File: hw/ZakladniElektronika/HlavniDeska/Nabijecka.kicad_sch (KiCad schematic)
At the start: 1 part

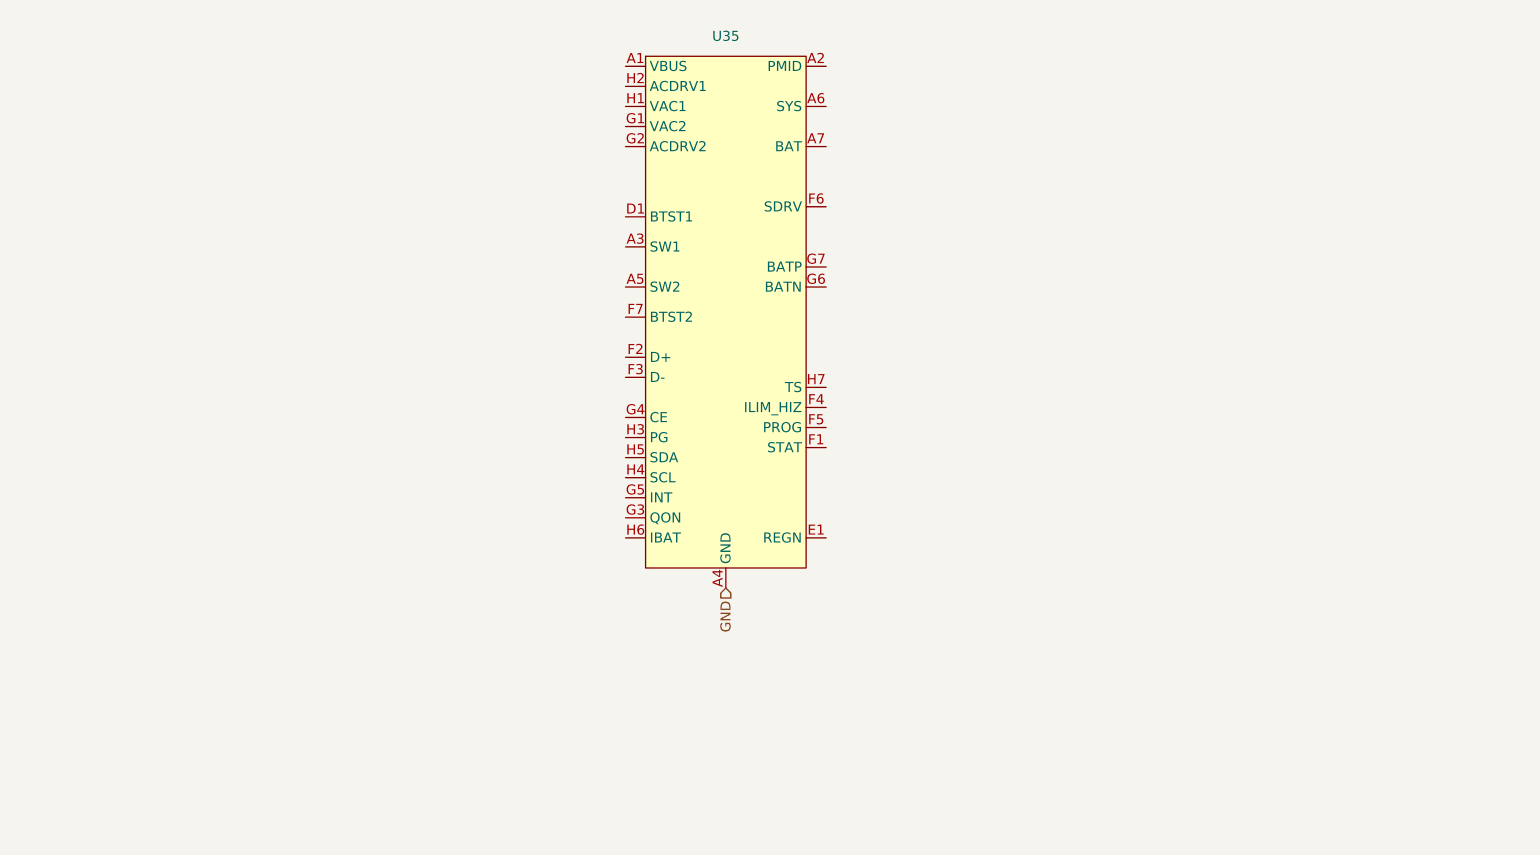
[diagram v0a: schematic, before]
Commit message: WIP
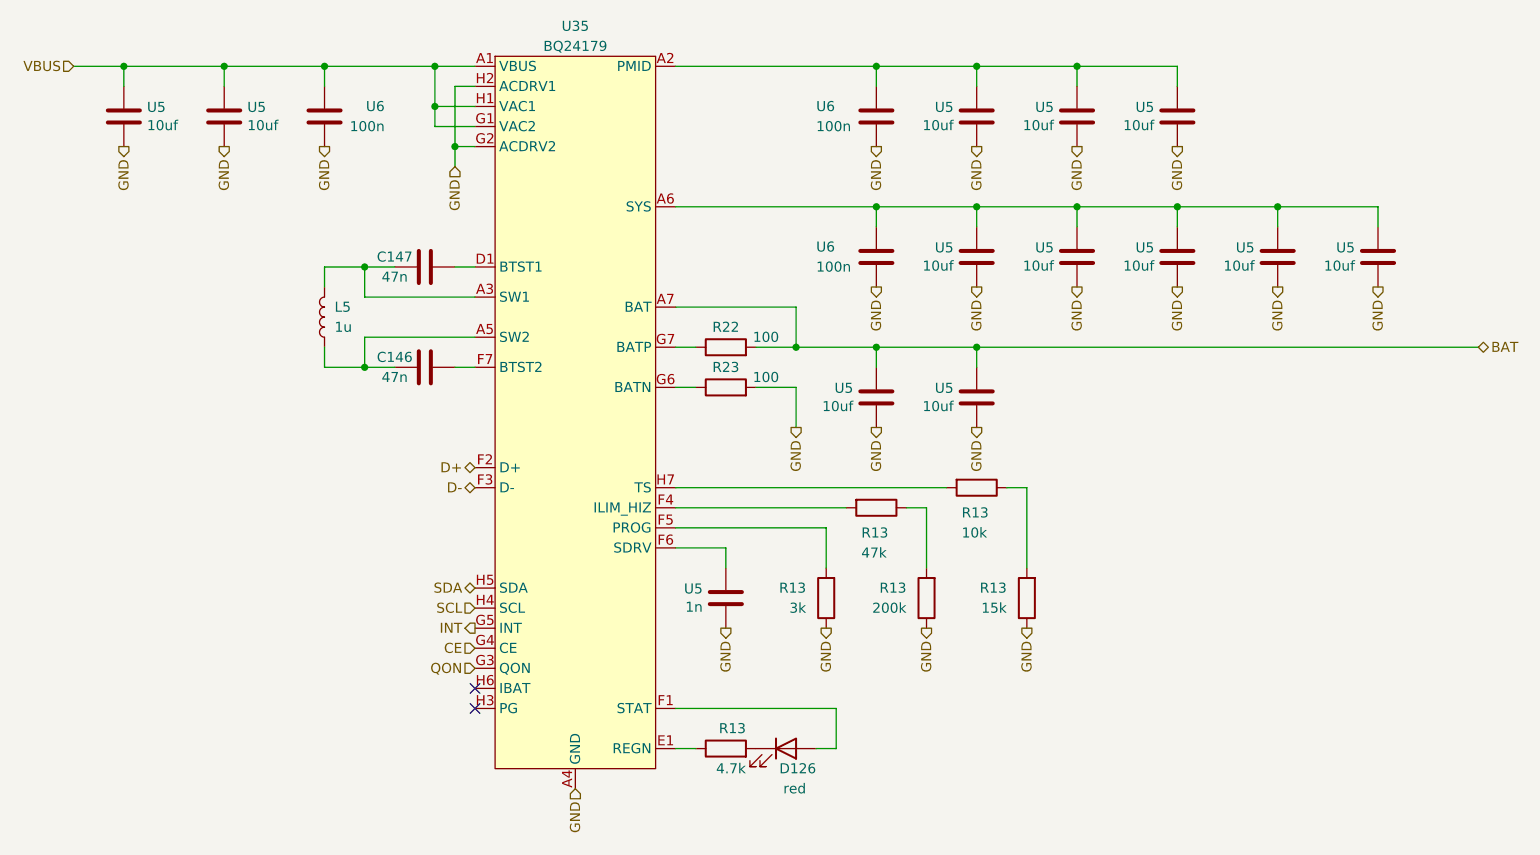
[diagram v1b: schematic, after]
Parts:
- added C146, C147: 47n, Capacitor_SMD:C_0402_1005Metric, symbol Device:C
- added D126: red, LED_SMD:LED_0603_1608Metric, symbol Device:LED
- added L5: 1u, Robotarna_KiCad_Library:SMD,4.2x4.4mm, symbol Device:L
- added R13: 4.7k, Resistor_SMD:R_0201_0603Metric, symbol Device:R
- added R13: 200k, Resistor_SMD:R_0402_1005Metric, symbol Device:R
- added R13: 10k, Resistor_SMD:R_0402_1005Metric, symbol Device:R
- added R13: 3k, Resistor_SMD:R_0402_1005Metric, symbol Device:R
- added R13: 47k, Resistor_SMD:R_0402_1005Metric, symbol Device:R
- added R13: 15k, Resistor_SMD:R_0402_1005Metric, symbol Device:R
- added R22, R23: 100, Resistor_SMD:R_0402_1005Metric, symbol Device:R
- added U5 (x12): 10uf, Capacitor_SMD:C_0805_2012Metric, symbol B.B-rescue:C-Device-B.B-rescue-B.B-rescue
- added U5: 1n, Capacitor_SMD:C_0402_1005Metric, symbol B.B-rescue:C-Device-B.B-rescue-B.B-rescue
- added U6 (x3): 100n, Capacitor_SMD:C_0402_1005Metric, symbol B.B-rescue:C-Device-B.B-rescue-B.B-rescue
- U35: value ~ -> BQ24179
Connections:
- net GMD: now also U35.G2 (ACDRV2), U35.H2 (ACDRV1), R13.1, R13.1, R13.1, R23.2, U5.2, U5.2, U5.2, U5.2, U5.2, U5.2, U5.2, U5.2, U5.2, U5.2, U5.2, U5.2, U5.2, U6.2, U6.2, U6.2
- net PMID: now also U5.1, U5.1, U5.1, U6.1
- net SW1: now also C147.1, L5.2
- net SW2: now also C146.1, L5.1
- net VBUS: now also U35.G1 (VAC2), U35.H1 (VAC1), U5.1, U5.1, U6.1
- net at U35.A6 (SYS), U35.B6 (SYS), U35.C6 (SYS)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: now also U5.1, U5.1, U5.1, U5.1, U5.1, U6.1
- net BAT: now reaches U35.A7 (BAT), U35.B7 (BAT), U35.C7 (BAT), U35.D7 (BAT), U35.E7 (BAT)
- net BAT: now also R22.2, U5.1, U5.1
- net at U35.D1 (BTST1): now also C147.2
- net at U35.E1 (REGN): now also R13.1
- net at U35.F1 (STAT): now also D126.2 (A)
- net D+: now reaches U35.F2 (D+)
- net D-: now reaches U35.F3 (D-)
- net at U35.F4 (ILIM_HIZ): now also R13.2
- net at U35.F5 (PROG): now also R13.2
- net at U35.F6 (SDRV): now also U5.1
- net at U35.F7 (BTST2): now also C146.2
- net QON: now reaches U35.G3 (QON)
- net CE: now reaches U35.G4 (CE)
- net INT: now reaches U35.G5 (INT)
- net at U35.G6 (BATN): now also R23.1
- net at U35.G7 (BATP): now also R22.1
- net SCL: now reaches U35.H4 (SCL)
- net SDA: now reaches U35.H5 (SDA)
- net at U35.H7 (TS): now also R13.2
- new net: D126.1 (K), R13.2
- new net: R13.1, R13.2 (x2)
- no-connect marks 0 -> 2
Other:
- moved on the sheet: U35

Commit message: Zaciame psat
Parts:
- U35: LCSC (none) -> C2879484
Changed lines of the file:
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@@
       (effects (font (size 1.27 1.27)) hide)
     )
-    (property "Datasheet" "" (at 133.35 50.8 0)
+    (property "Datasheet" "https://www.ti.com/lit/ds/symlink/bq24179.pdf?ts=1698854511988&ref_url=https%253A%252F%252Fwww.ti.com%252Fpower-management%252Fbattery-management%252Fcharger-ics%252Fproducts.html" (at 133.35 50.8 0)
       (effects (font (size 1.27 1.27)) hide)
     )
+    (property "LCSC" "C2879484" (at 133.35 50.8 0)
+      (effects (font (size 1.27 1.27)) hide)
+    )

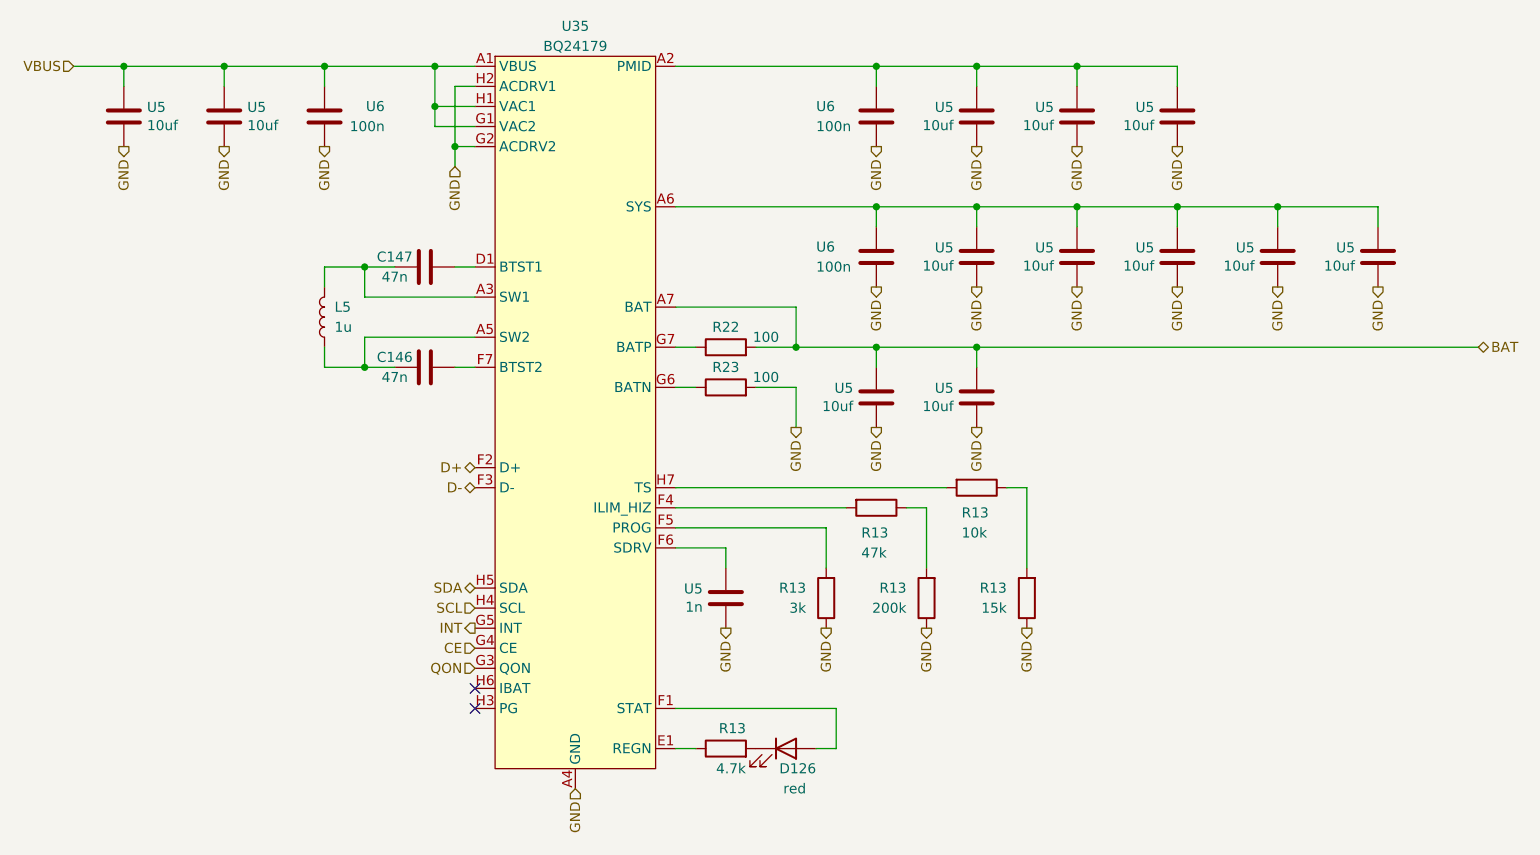
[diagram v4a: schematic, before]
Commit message: USB_multiplexer a přehlednost
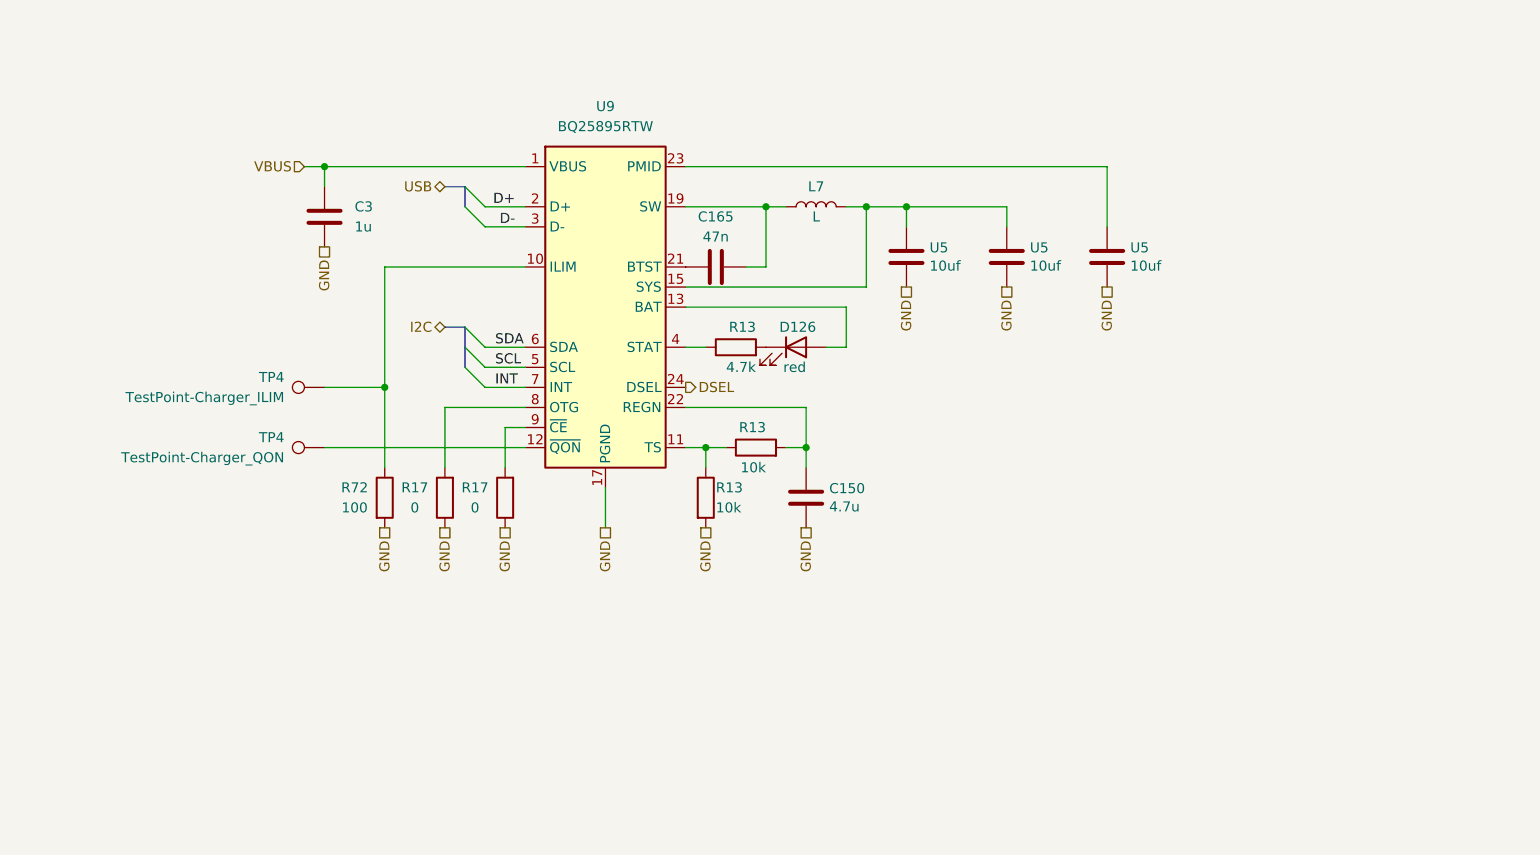
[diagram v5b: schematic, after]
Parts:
- removed C146, C147: 47n, Capacitor_SMD:C_0402_1005Metric, symbol Device:C
- removed L5: 1u, Robotarna_KiCad_Library:SMD,4.2x4.4mm, symbol Device:L
- removed R13: 4.7k, Resistor_SMD:R_0201_0603Metric, symbol Device:R
- removed R13: 200k, Resistor_SMD:R_0402_1005Metric, symbol Device:R
- removed R13: 10k, Resistor_SMD:R_0402_1005Metric, symbol Device:R
- removed R13: 3k, Resistor_SMD:R_0402_1005Metric, symbol Device:R
- removed R13: 47k, Resistor_SMD:R_0402_1005Metric, symbol Device:R
- removed R13: 15k, Resistor_SMD:R_0402_1005Metric, symbol Device:R
- removed R22, R23: 100, Resistor_SMD:R_0402_1005Metric, symbol Device:R
- removed U35: BQ24179, symbol Robotarna_KiCad_Library:BQ24179
- removed U5 (x12): 10uf, Capacitor_SMD:C_0805_2012Metric, symbol B.B-rescue:C-Device-B.B-rescue-B.B-rescue
- removed U5: 1n, Capacitor_SMD:C_0402_1005Metric, symbol B.B-rescue:C-Device-B.B-rescue-B.B-rescue
- removed U6 (x3): 100n, Capacitor_SMD:C_0402_1005Metric, symbol B.B-rescue:C-Device-B.B-rescue-B.B-rescue
- added C150: 4.7u, Capacitor_SMD:C_0805_2012Metric, symbol Device:C
- added C165: 47n, Capacitor_SMD:C_0402_1005Metric, symbol Device:C
- added C3: 1u, Capacitor_SMD:C_0402_1005Metric, symbol Device:C
- added L7: L, Inductor_SMD:L_Abracon_ASPI-0630LR, symbol Device:L
- added R13: 4.7k, Resistor_SMD:R_0201_0603Metric, symbol Device:R
- added R13 (x2): 10k, Resistor_SMD:R_0402_1005Metric, symbol Device:R
- added R17 (x2): 0, Resistor_SMD:R_0805_2012Metric_Pad1.20x1.40mm_HandSolder, symbol Device:R
- added R72: 100, Resistor_SMD:R_0402_1005Metric, symbol Device:R
- added TP4: TestPoint-Charger_QON, symbol Connector:TestPoint
- added TP4: TestPoint-Charger_ILIM, symbol Connector:TestPoint
- added U5 (x3): 10uf, Capacitor_SMD:C_0805_2012Metric, symbol B.B-rescue:C-Device-B.B-rescue-B.B-rescue
- added U9: BQ25895RTW, Package_DFN_QFN:Texas_S-PWQFN-N24_EP2.7x2.7mm_ThermalVias, symbol Battery_Management:BQ25895RTW
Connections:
- net D+: now also U9.2 (D+)
- net D-: now also U9.3 (D-)
- net INT: now also U9.7 (INT)
- net SCL: now also U9.5 (SCL)
- net SDA: now also U9.6 (SDA)
- net VBUS: now also C3.1, U9.1 (VBUS)
- net at D126.1 (K): now also R13.2
- net at D126.2 (A): now also U9.13 (BAT), U9.14 (BAT)
- new net: U5.1, U9.23 (PMID)
- new net: C165.1, L7.1, U9.19 (SW), U9.20 (SW)
- new net: C165.2, U9.21 (BTST)
- new net: C150.1, R13.2, U9.22 (REGN)
- new net: L7.2, U5.1, U5.1, U9.15 (SYS), U9.16 (SYS)
- new net: TP4.1, U9.12 (~{QON})
- new net: R17.2, U9.8 (OTG)
- new net: R17.2, U9.9 (~{CE})
- new net: R72.1, TP4.1, U9.10 (ILIM)
- new net: R13.1, U9.4 (STAT)
- new net: R13.1, R13.1, U9.11 (TS)
- new net DSEL: U9.24 (DSEL)
- new net GND: C150.2, C3.2, R13.2, R17.1, R17.1, R72.2, U5.2, U5.2, U5.2, U9.17 (PGND), U9.18 (PGND), U9.25 (PGND)
- no-connect marks 2 -> 0
